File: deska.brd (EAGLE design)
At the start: 100 x 80 mm, 18 parts, among them Q1 BC547, Q2 BC547

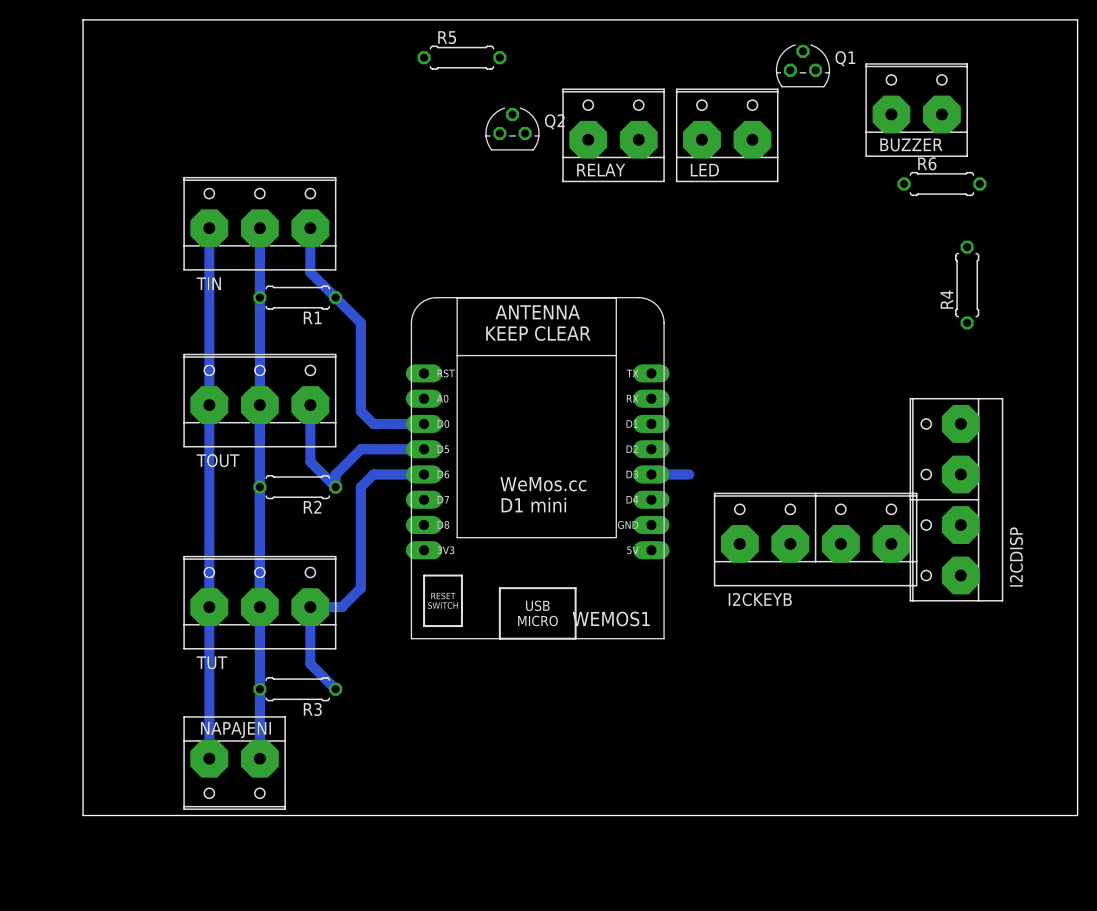
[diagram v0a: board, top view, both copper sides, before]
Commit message: upravy desky
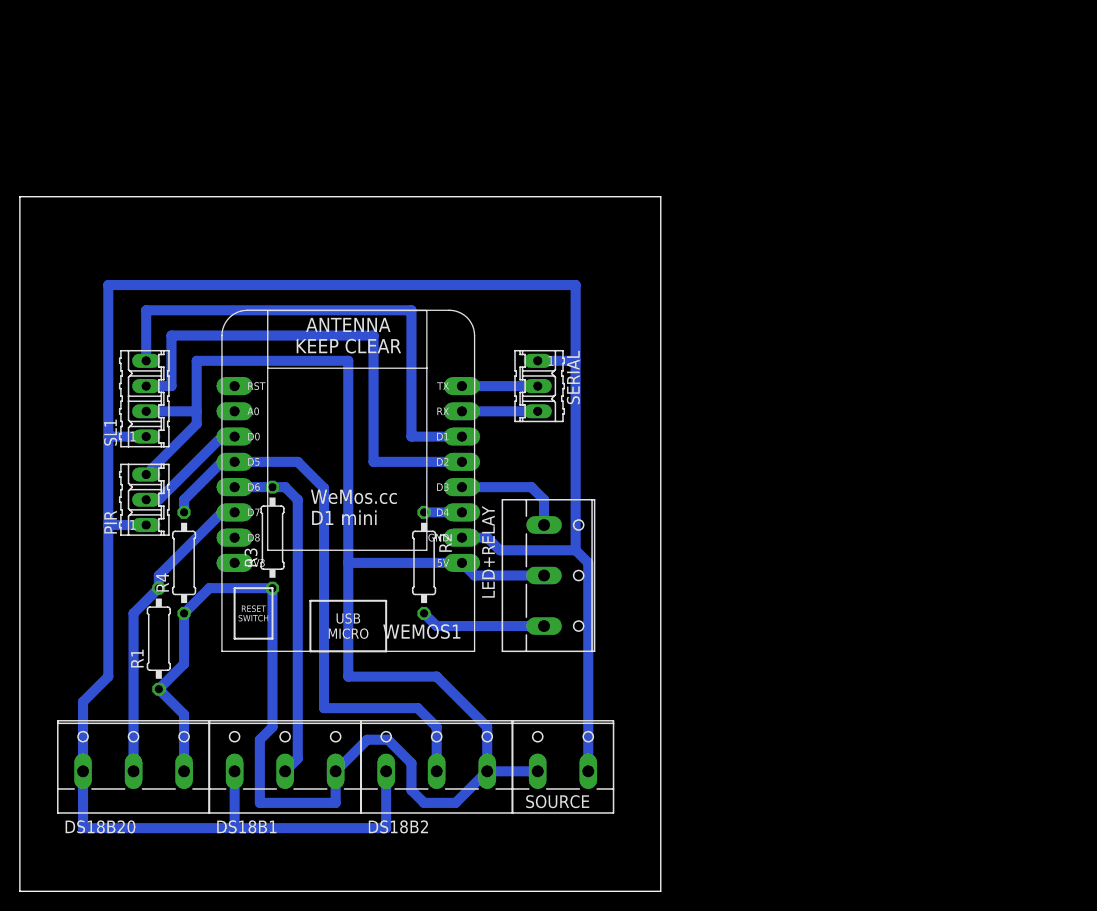
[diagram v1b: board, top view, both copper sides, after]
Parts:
- removed BUZZER, LED, NAPAJENI, RELAY: (no value), con-wago-508:W237-132
- removed I2CDISP, I2CKEYB: (no value), con-wago-508:W237-4P
- removed Q1, Q2: BC547, transistor-npn:TO92
- removed R5, R6: 1k, rcl:0207/7
- removed TIN, TOUT, TUT: (no value), con-wago-508:W237-3E
- added DS18B1, DS18B2, DS18B20, LED+RELAY: (no value), con-wago-508:W237-133
- added PIR, SERIAL: (no value), con-amp-quick:03P
- added SL1: (no value), con-amp-quick:04P
- added SOURCE: (no value), con-wago-508:W237-132
- R1, R3: device rcl:0207/7 -> rcl:0207/10
- R2: value 4k7 -> 220; device rcl:0207/7 -> rcl:0207/10
- R4: value 220 -> 4k7; device rcl:0207/7 -> rcl:0207/10
- WEMOS1: device wemos:WEMOS-D1-MINI -> esp8266modules:WEMOS-D1-MINI
- moved R4 83.6 mm to (10.2, 25.4)
- moved R1 37.0 mm to (7.62, 17.8), turned to 90 degrees
- moved WEMOS1 19.1 mm to (25.4, 35.6)
- moved R3 15.5 mm to (19.1, 27.9), turned to 90 degrees
- moved R2 14.8 mm to (34.3, 25.4), turned to 270 degrees
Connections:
- removed net N$12: I2CDISP.3, I2CKEYB.3, WEMOS1.D4
- removed net N$14: Q2.3, RELAY.1
- removed net N$15: BUZZER.1, Q1.3
- removed net N$16: R6.2, WEMOS1.D2
- removed net N$19: R2.1, TOUT.3, WEMOS1.D5
- new net N$2: SERIAL.3, WEMOS1.RX
- new net N$8: LED+RELAY.3, R2.2
- new net N$9: DS18B20.2, R1.2, WEMOS1.D7
- net +5V: now also DS18B1.3, DS18B2.3, DS18B20.3, LED+RELAY.2, PIR.3, R1.1, R3.1, R4.1, SL1.2, SOURCE.1; no longer I2CDISP.2, I2CKEYB.2, LED.2, NAPAJENI.1, R1.2, R2.2, R3.2, RELAY.2, TIN.2, TOUT.2, TUT.2
- net GND: now also DS18B1.1, DS18B2.1, DS18B20.1, PIR.1, SERIAL.1, SL1.1, SOURCE.2; no longer BUZZER.2, I2CDISP.1, I2CKEYB.1, NAPAJENI.2, Q1.1, Q2.1, TIN.1, TOUT.1, TUT.1
- net N$1: now also SERIAL.2, WEMOS1.TX; no longer R1.1, TIN.3, WEMOS1.D0
- net N$11: now also DS18B2.2, R4.2, WEMOS1.D5; no longer I2CDISP.4, I2CKEYB.4, WEMOS1.D3
- net N$13: now also DS18B1.2, R3.2, WEMOS1.D6; no longer Q2.2, R5.2
- net N$3: now also SL1.4, WEMOS1.D1; no longer R3.1, TUT.3, WEMOS1.D6
- net N$4: now also SL1.3, WEMOS1.D2; no longer R5.1, WEMOS1.D7
- net N$5: now also PIR.2, WEMOS1.D0; no longer R4.1, WEMOS1.D8
- net N$6: now also R2.1, WEMOS1.D4; no longer LED.1, R4.2
- net N$7: now also LED+RELAY.1, WEMOS1.D3; no longer Q1.2, R6.1
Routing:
- net GND: track 53.3 -> 217.4 mm
- net +5V: track 73.7 -> 194.3 mm
- net N$11: track 3.81 -> 56.7 mm
- net N$4: track 0.00 -> 49.5 mm
- net N$13: track 0.00 -> 34.7 mm
- net N$9: track 0.00 -> 31.0 mm
- net N$19: track 20.5 -> 0.00 mm
- net N$1: track 27.4 -> 7.62 mm
- net N$3: track 32.2 -> 49.5 mm
- net N$8: track 0.00 -> 12.6 mm
- net N$5: track 0.00 -> 11.5 mm
- net N$7: track 0.00 -> 11.3 mm
- net N$2: track 0.00 -> 7.62 mm
- net N$6: track 0.00 -> 3.81 mm
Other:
- board size 100 x 80 mm -> 64.4 x 69.8 mm
